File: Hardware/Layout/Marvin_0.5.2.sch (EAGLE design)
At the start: 56 parts, among them IC1 LM321MF, Q1 IRLML5203, Q2 IRLML5203, Q3 IRLML5203, U1 ATMEGA32U4-XUAU, U2 SI2366DS-T1-GE3, U3 SI2366DS-T1-GE3, U4 SI2366DS-T1-GE3, U5 LT1761IS5-3.3TRMPBF, X3 BU-SMA-H, Y1 CSTCE16M0V53-R0 16MHZ

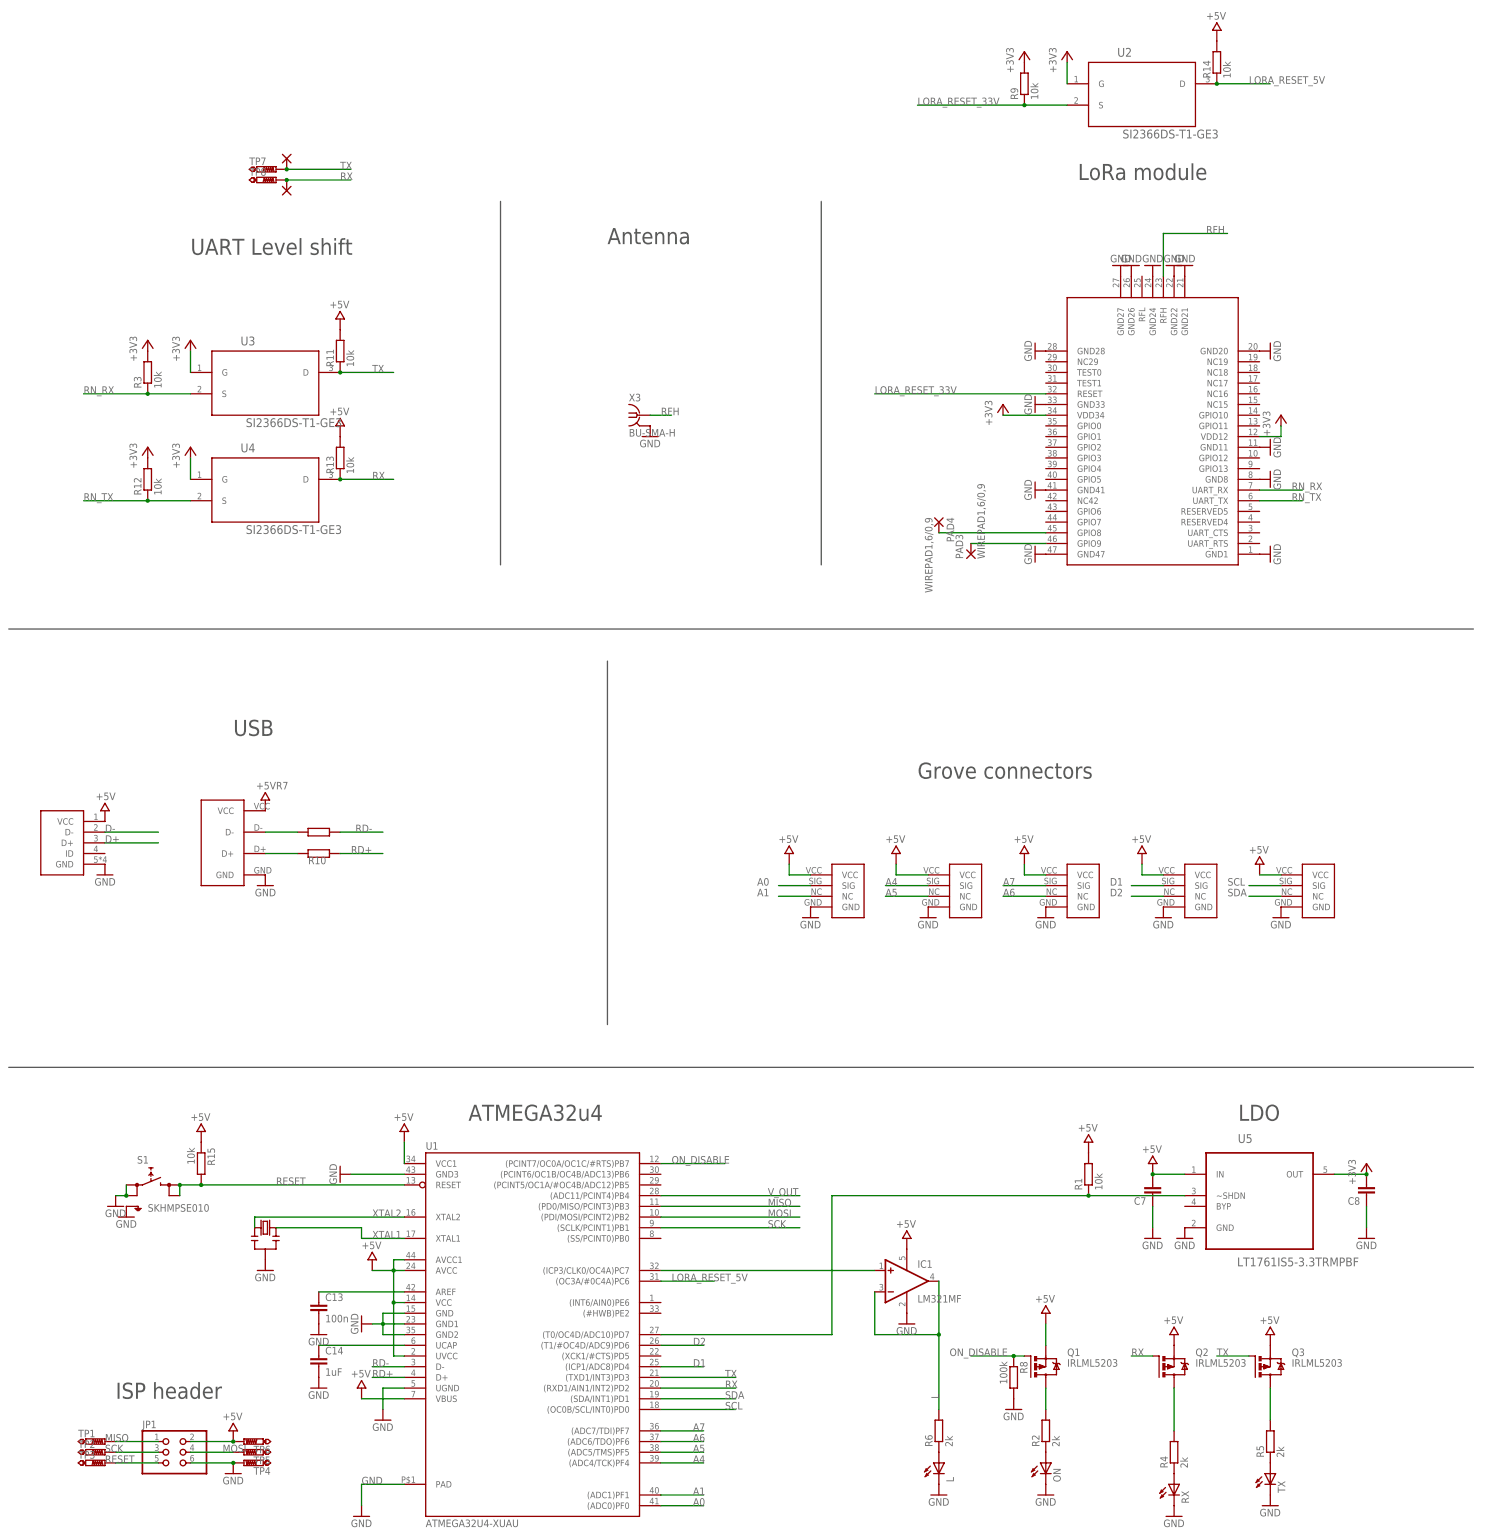
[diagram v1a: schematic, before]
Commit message: cleaning up pcb
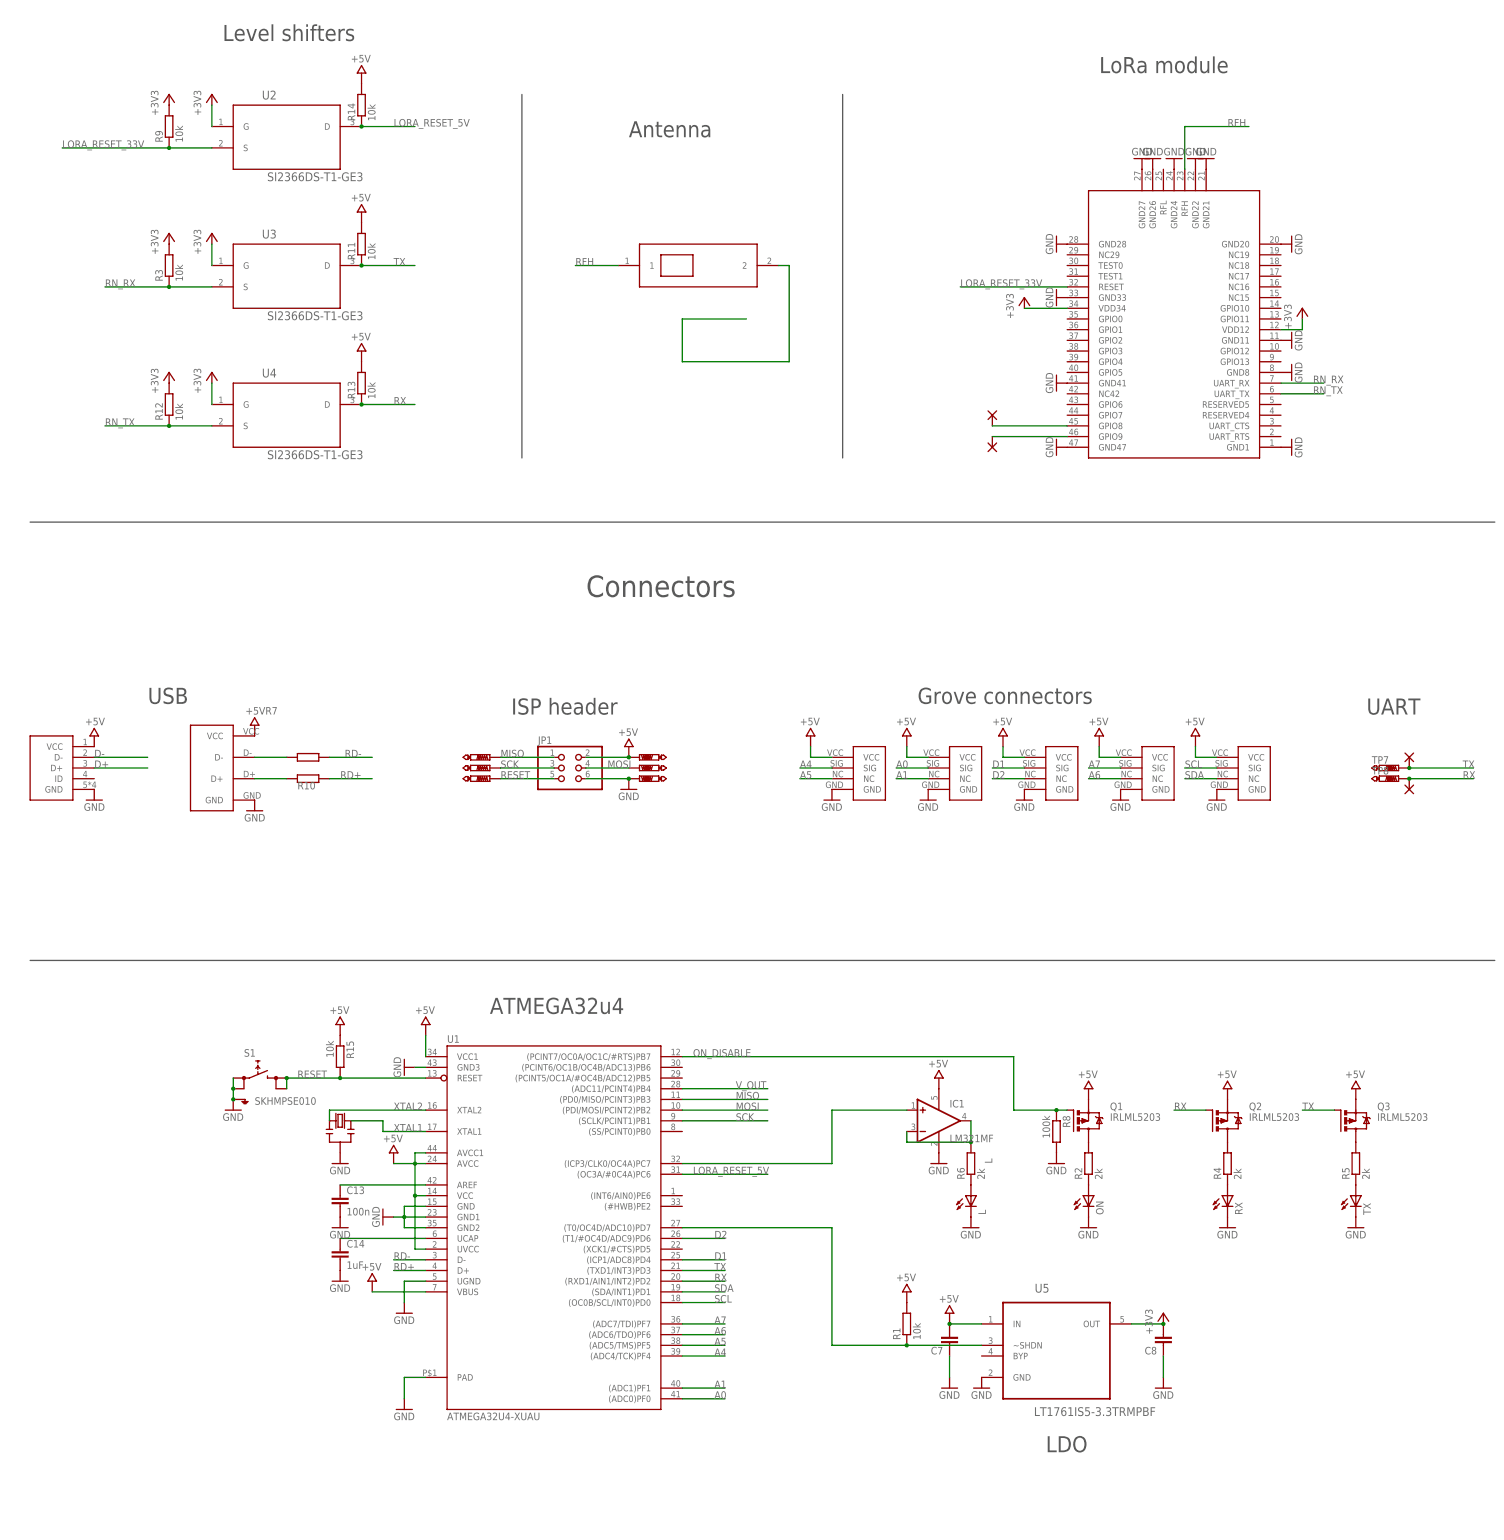
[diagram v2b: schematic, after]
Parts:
- removed X3: BU-SMA-H, con-coax:BU-SMA-H
- added U$25: 868AT, 868AT43_antenna:868AT
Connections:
- new net N$13: U$25.2
- net GND: no longer X3.2
- net RFH: now also U$25.1; no longer X3.1
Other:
- note added: "Connectors"
- note added: "Level shifters"
- note added: "UART"
- note removed: "UART Level shift"
- moved on the sheet: C13, C14, C7, C8, IC1, JP1, L, ON, Q1, Q2, Q3, R1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
